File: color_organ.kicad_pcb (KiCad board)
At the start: 2 copper layers, 110.2 x 116.8 mm, 125 parts, among them CON1 BARREL_JACK, J1 Audio_3.5mm, Q1 2N3904, Q2 2N3904, Q3 2N3904, Q4 2N3904, Q5 2N3904, Q6 2N3904, SW1 SPST, U1 MC33204P, U2 MC33204P, U3 MC34072P

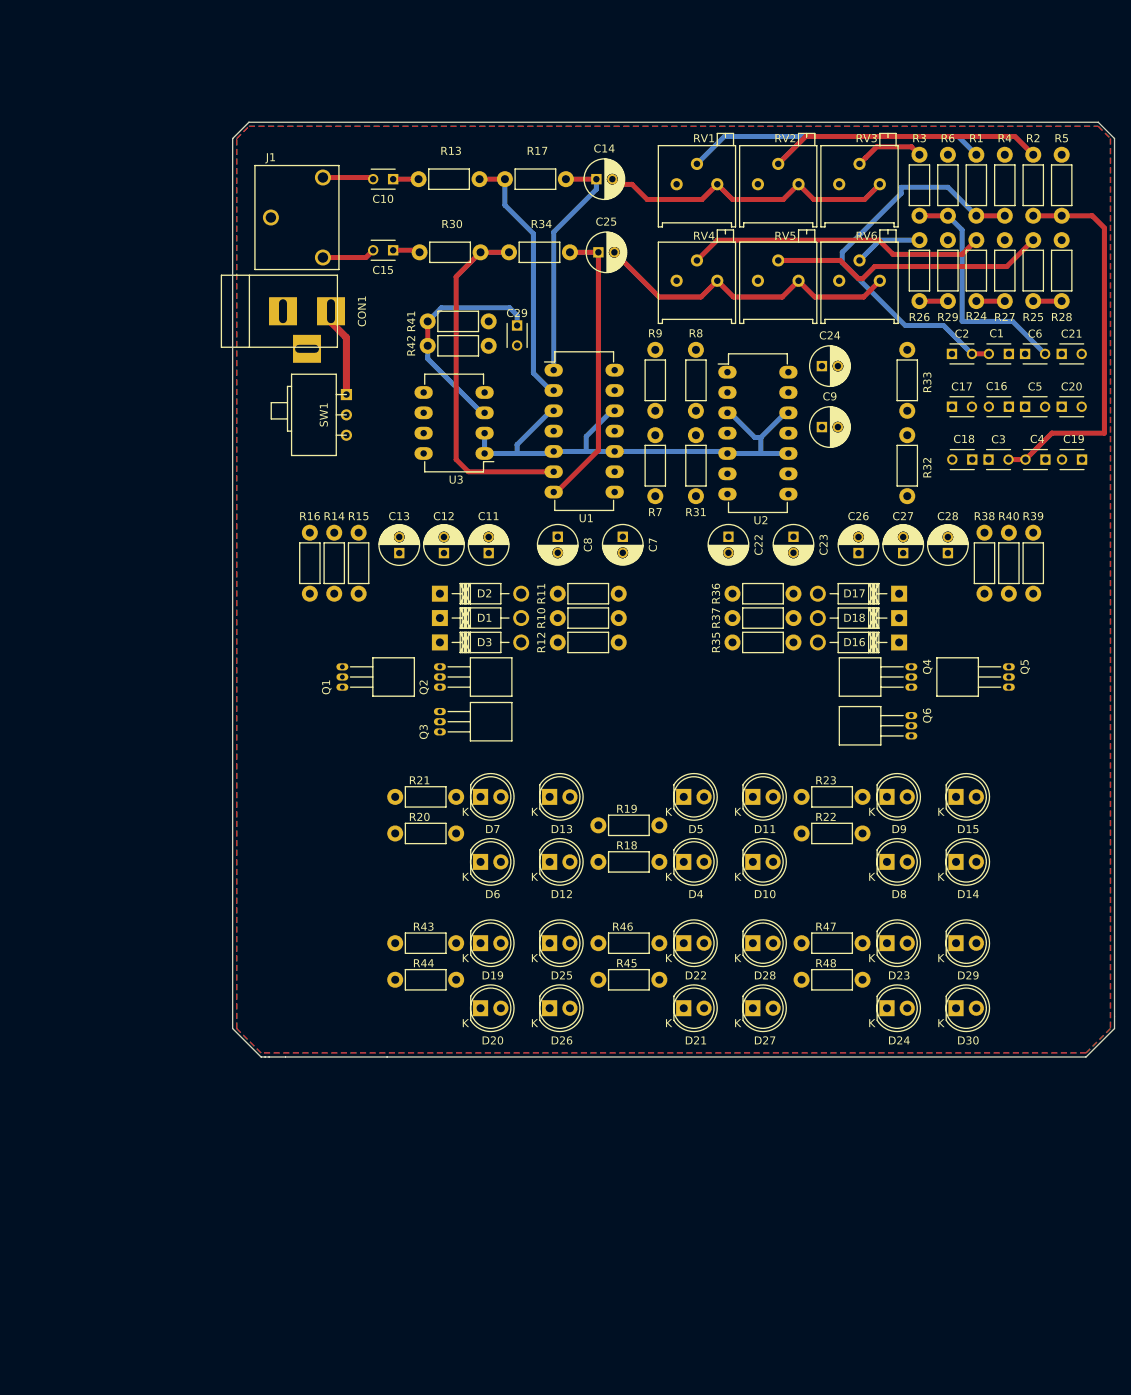
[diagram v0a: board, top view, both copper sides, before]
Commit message: Initial board design done.
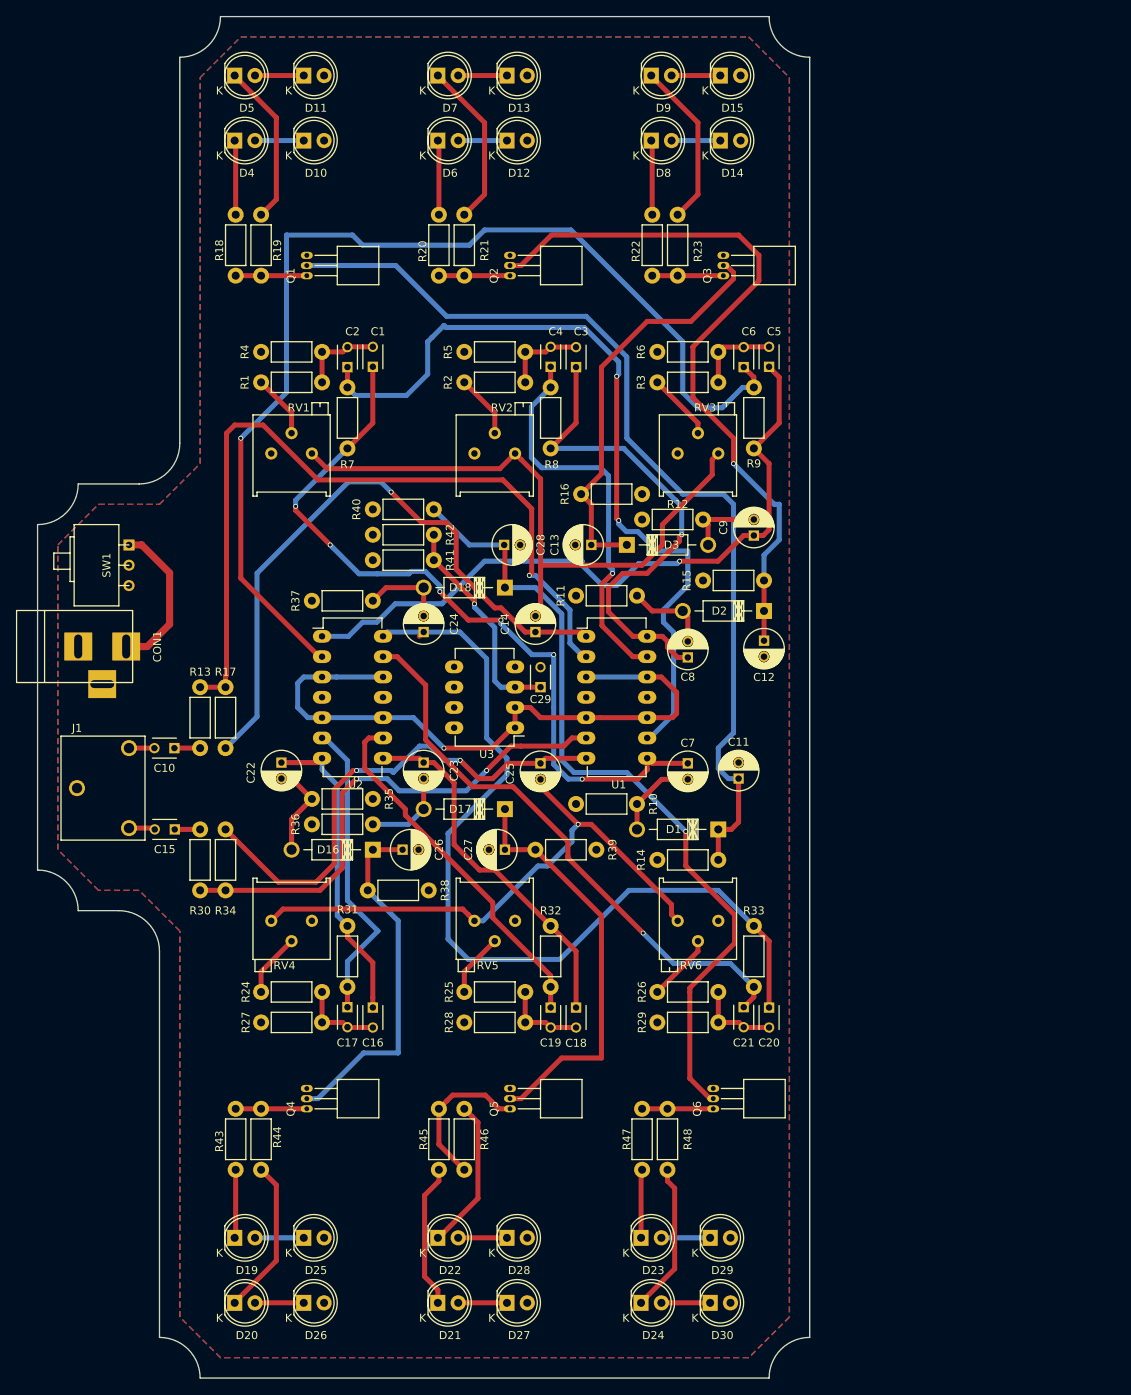
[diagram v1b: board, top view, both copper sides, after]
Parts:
- moved R27 134.9 mm to (55.9, 146.1), turned to 0 degrees
- moved R24 129.7 mm to (55.9, 142.2), turned to 0 degrees
- moved R28 123.0 mm to (81.3, 146.1), turned to 0 degrees
- moved R25 117.9 mm to (81.3, 142.2), turned to 0 degrees
- moved C16 109.4 mm to (69.8, 144.2), turned to 270 degrees
- moved C17 106.5 mm to (66.7, 144.1), turned to 270 degrees
- moved D10 106.2 mm to (61.2, 35.8)
- moved D11 106.2 mm to (61.2, 27.7)
- moved D4 106.2 mm to (52.6, 35.8)
- moved D5 106.2 mm to (52.6, 27.7)
- moved R29 104.3 mm to (105.4, 146.1), turned to 0 degrees
- moved R26 99.5 mm to (105.4, 142.2), turned to 0 degrees
- moved RV4 97.5 mm to (57.1, 133.3), turned to 180 degrees
- moved R18 96.7 mm to (52.7, 45.1), turned to 270 degrees
- moved R4 96.2 mm to (55.9, 62.2), turned to 0 degrees
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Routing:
- net Net-(C6-Pad1): track 0.00 -> 136.6 mm, vias 0 -> 1
- net Net-(C11-Pad1): track 0.00 -> 120.7 mm
- net Net-(C20-Pad1): track 0.00 -> 110.2 mm
- net Net-(C2-Pad1): track 0.00 -> 102.0 mm, vias 0 -> 2
- net Net-(C28-Pad1): track 0.00 -> 101.6 mm, vias 0 -> 1
- net Net-(C1-Pad1): track 0.00 -> 96.0 mm, vias 0 -> 6
- net Net-(C12-Pad1): track 0.00 -> 91.0 mm, vias 0 -> 1
- net Net-(C5-Pad1): track 0.00 -> 87.2 mm, vias 0 -> 1
- net Net-(C21-Pad1): track 0.00 -> 71.7 mm, vias 0 -> 1
- net Net-(R13-Pad2): track 32.8 -> 100.1 mm, vias 0 -> 1
- net Net-(C3-Pad1): track 0.00 -> 62.7 mm, vias 0 -> 1
- net Net-(C27-Pad1): track 0.00 -> 51.9 mm
- net Net-(C13-Pad1): track 0.00 -> 51.7 mm
- net Net-(C14-Pad1): track 29.9 -> 80.0 mm, vias 0 -> 1
- net Net-(C4-Pad1): track 0.00 -> 49.7 mm, vias 0 -> 1
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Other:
- board size 110.2 x 116.8 mm -> 96.5 x 170.2 mm
